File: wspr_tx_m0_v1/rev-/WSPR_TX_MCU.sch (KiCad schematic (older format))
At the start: 4 parts, among them J1 Conn_01x12_Male, J2 Conn_01x15_Male, U1 ATSAMD21G18A-AUT, Y1 Crystal_32k768

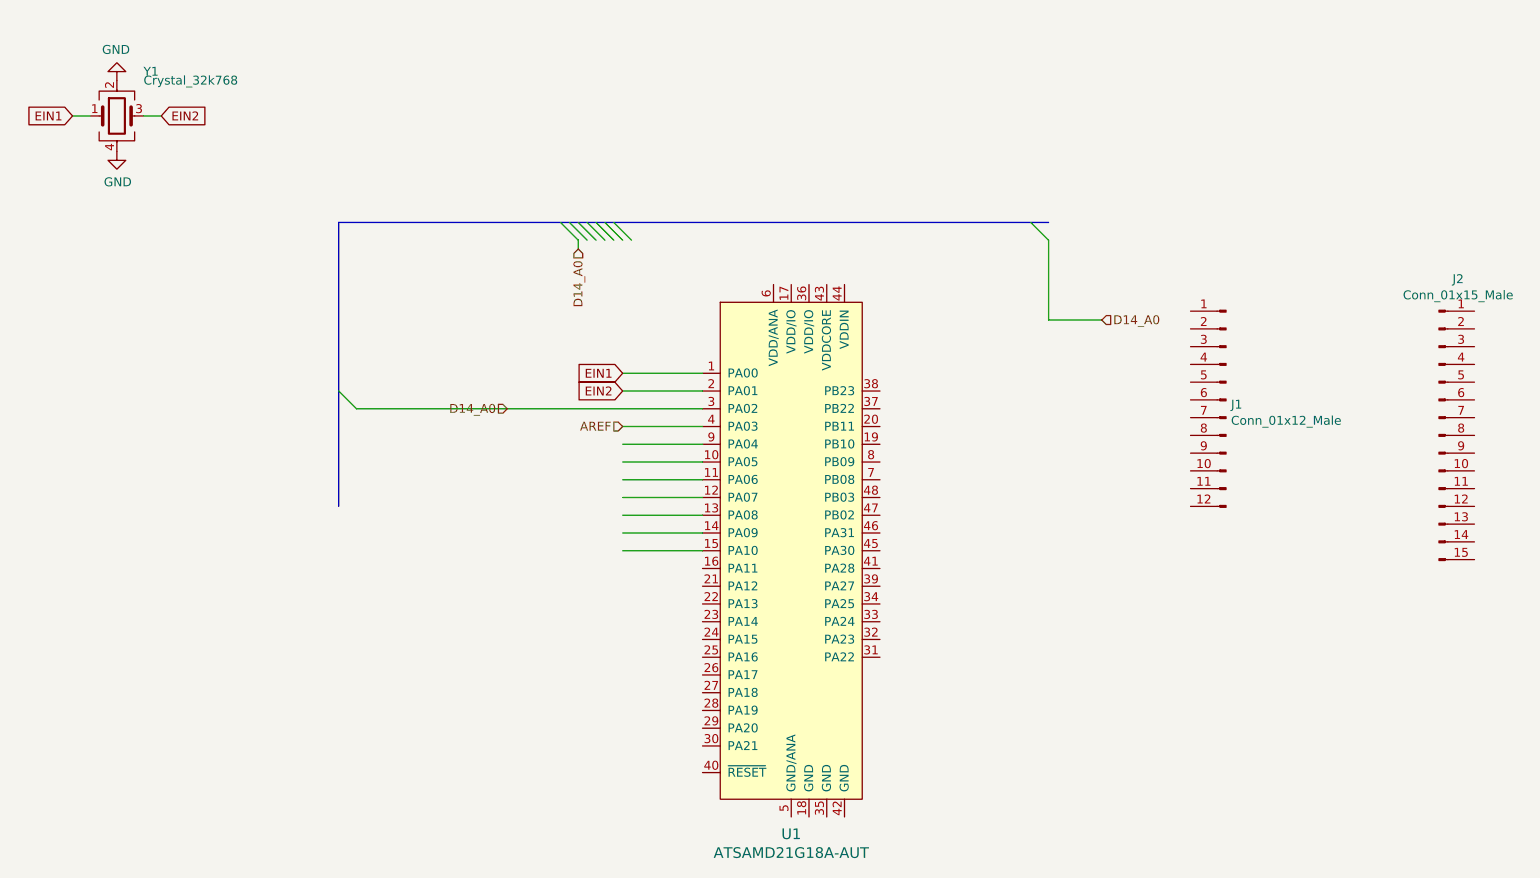
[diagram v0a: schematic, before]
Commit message: mass commit, lots of changes to m0 board, not functional yet.  added schematic for featherwinf in PDF form.
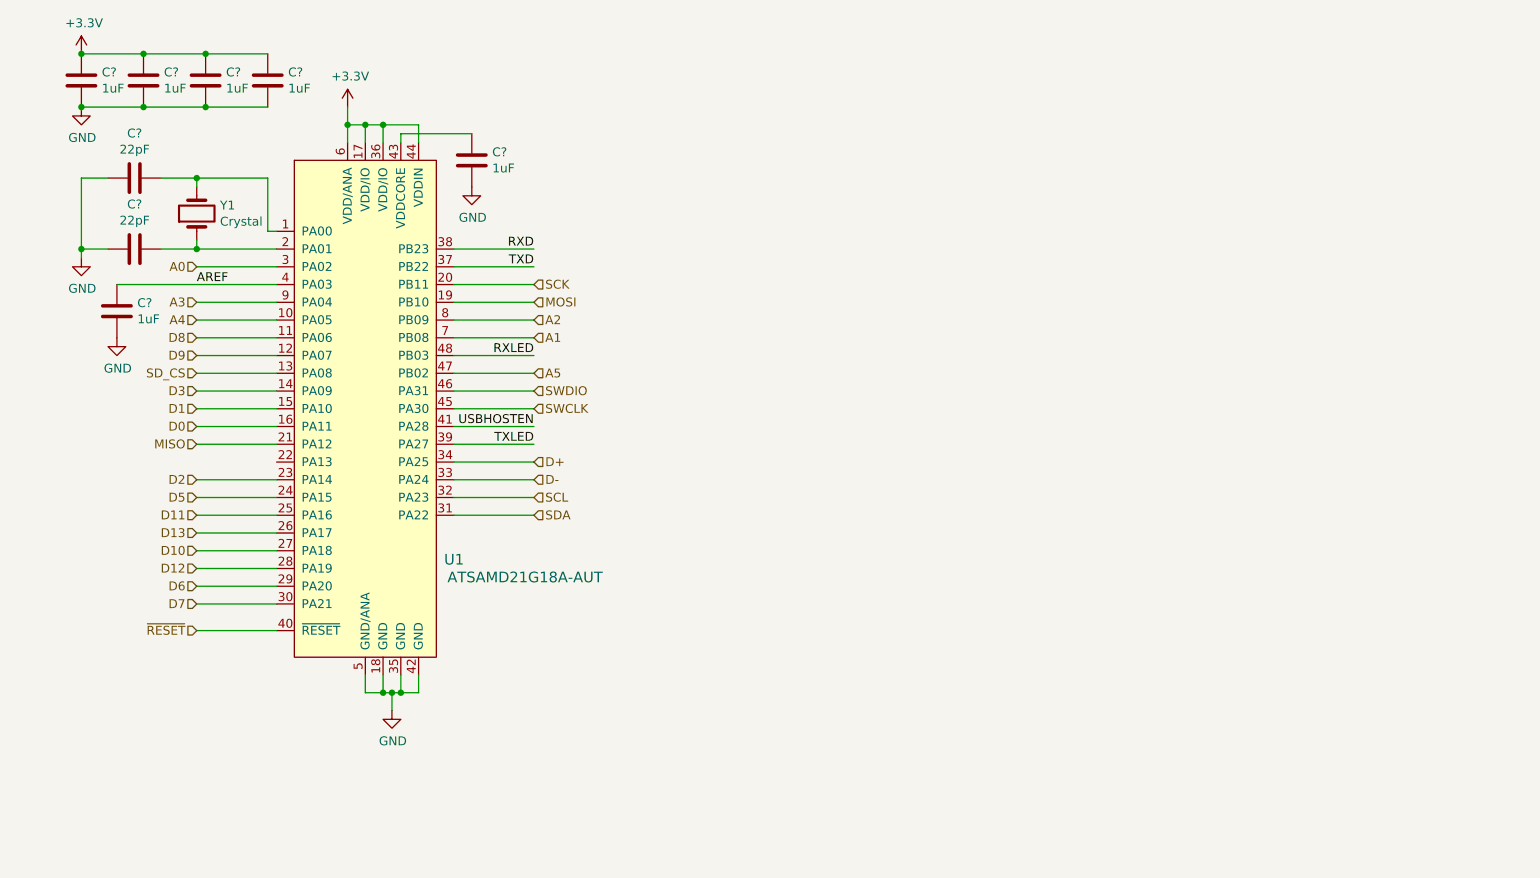
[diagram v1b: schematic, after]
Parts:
- removed J1: Conn_01x12_Male, symbol Connector:Conn_01x12_Male
- removed J2: Conn_01x15_Male, symbol Connector:Conn_01x15_Male
- removed Y1: Crystal_32k768, Crystal:Crystal_SMD_Abracon_ABM8G-4Pin_3.2x2.5mm, symbol Device:Crystal_GND24
- added C? (x6): 1uF, symbol Device:C
- added C? (x2): 22pF, symbol Device:C
- added Y1: Crystal, Crystal:Crystal_SMD_G8-2Pin_3.2x1.5mm_HandSoldering, symbol Device:Crystal
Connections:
- net labels added: +3.3V, A0, A1, A2, A3, A4, A5, D+, D-, D0, D1, D10, D11, D12, D13, D2, D3, D5, D6, D7, D8, D9, MISO, MOSI, RXD, RXLED, SCK, SCL, SDA, SD_CS, SWCLK, SWDIO, TXD, TXLED, USBHOSTEN, ~RESET
- net labels removed: D14_A0, EIN1, EIN2
- wire segments 16 -> 73
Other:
- moved on the sheet: U1
